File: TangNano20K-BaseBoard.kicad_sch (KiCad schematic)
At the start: 49 parts, among them J1 Conn_01x20_Socket, J2 Conn_01x20_Socket, J3 Conn_01x06_Socket, J4 Conn_01x06_Socket, Q1 PN2222A, Q2 PN2222A, Q3 PN2222A, Q4 PN2222A, SW1 SW_SPDT_321, SW2 SW_SPDT_321, SW3 SW_SPDT_321, SW4 SW_SPDT_321, SW5 SW_SPDT_321, U1 CC56-12EWA, U2 SSD1306

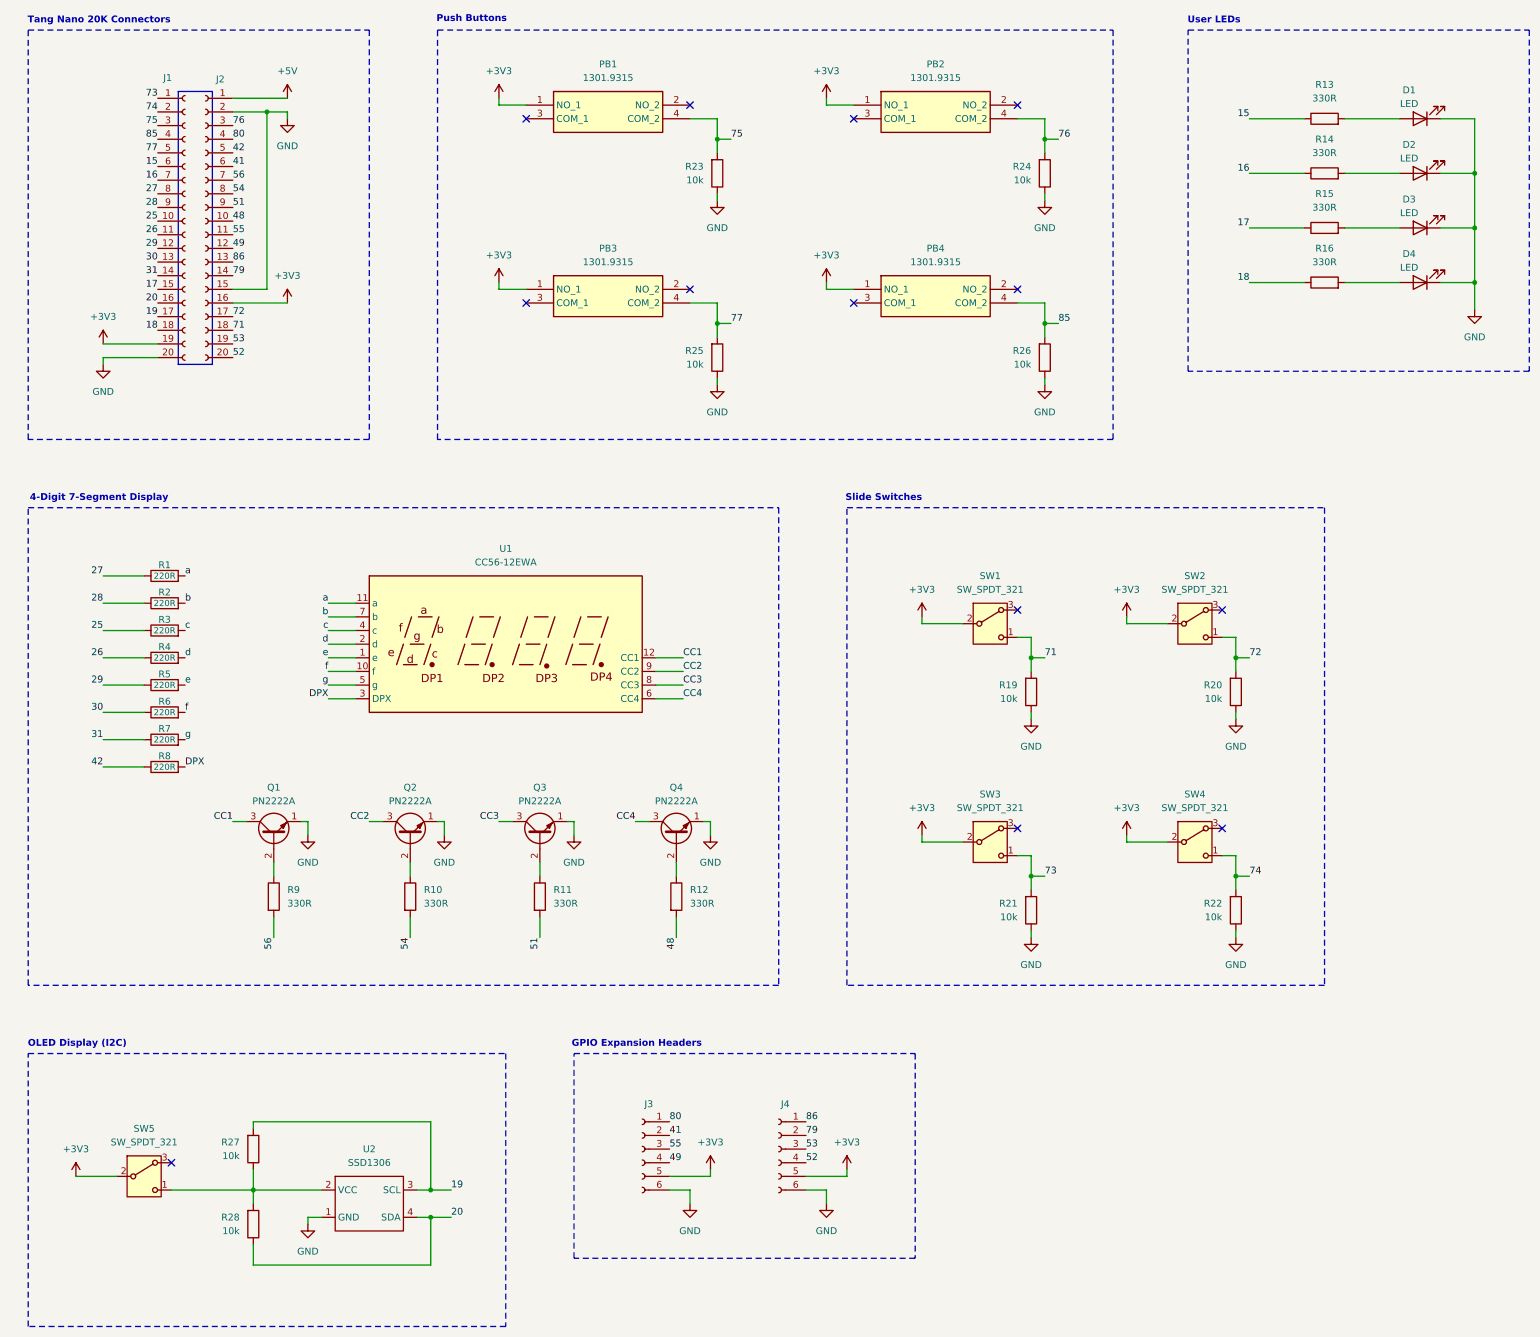
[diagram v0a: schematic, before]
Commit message: Update schematic and pcb
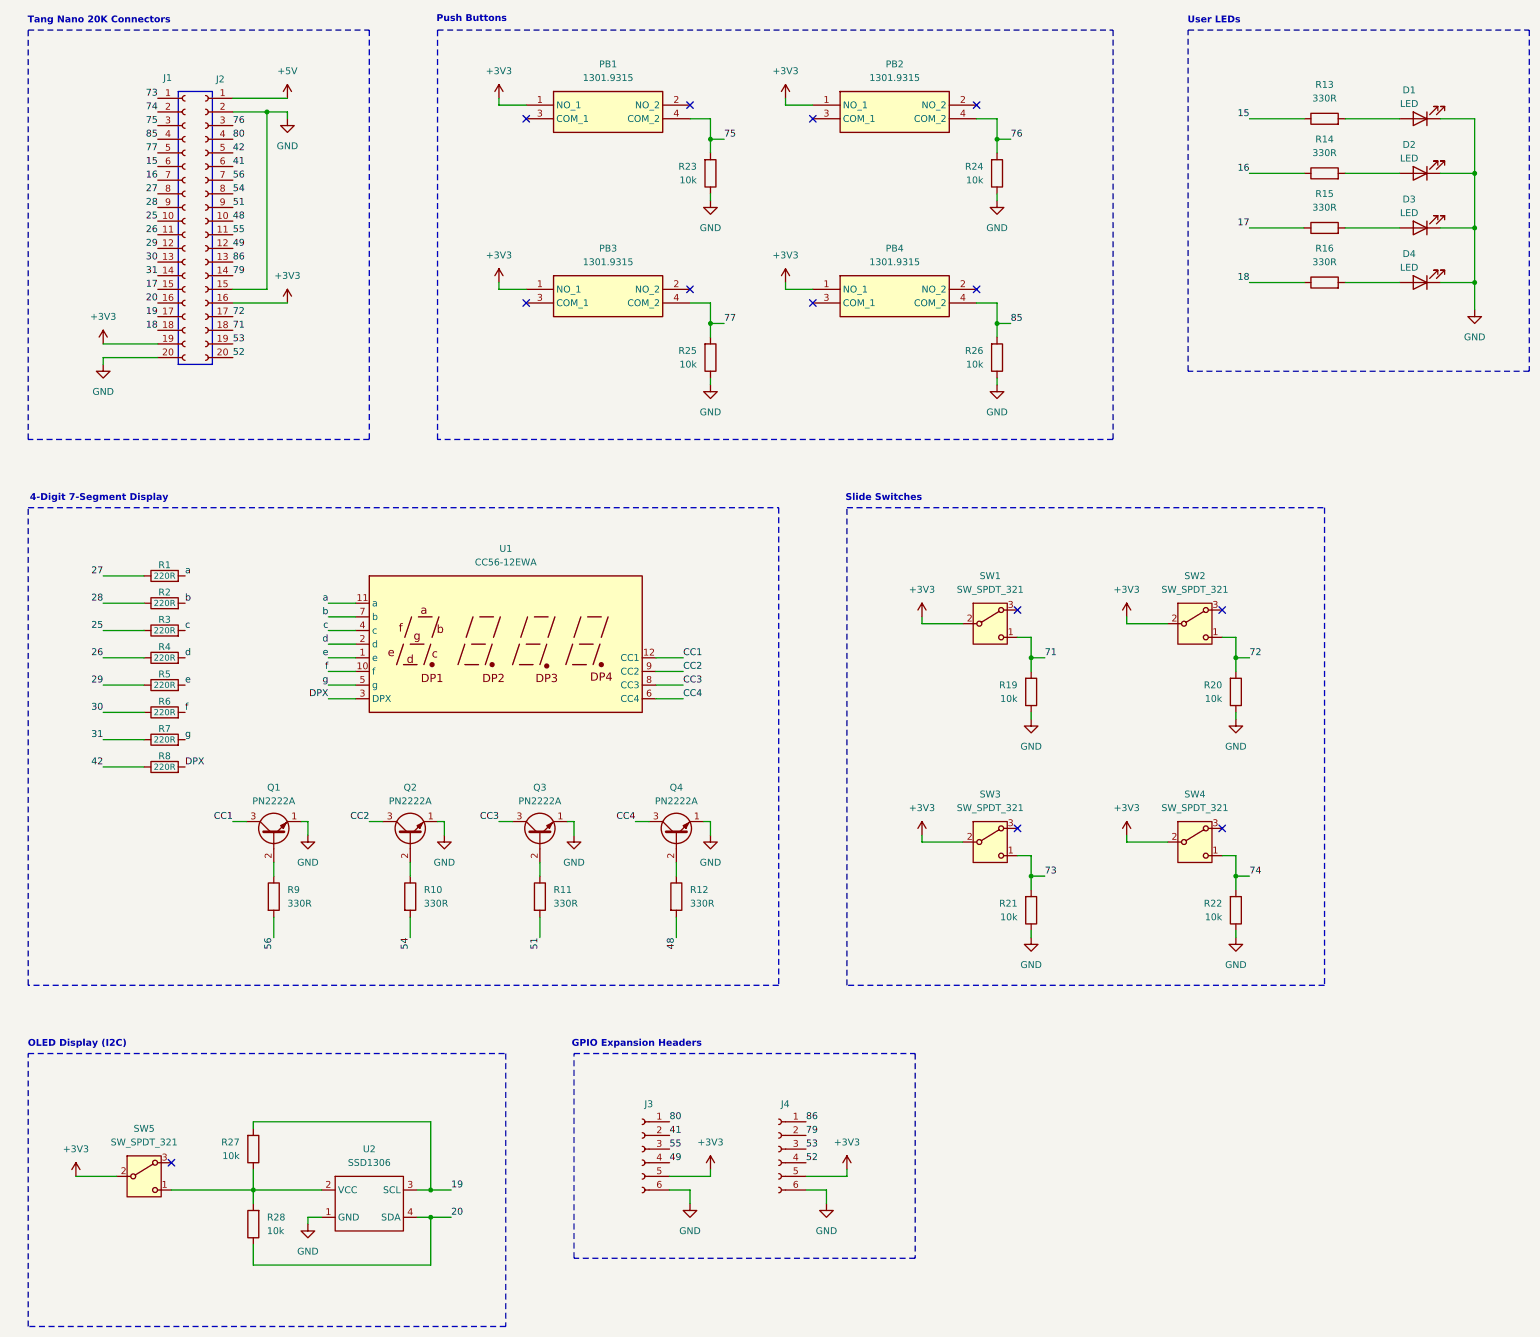
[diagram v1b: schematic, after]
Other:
- moved on the sheet: R23, R28
